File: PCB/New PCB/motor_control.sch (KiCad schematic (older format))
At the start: 29 parts, among them P4 CONN_2, P5 CONN_2, Q1 MOSFET_P, Q2 MOSFET_N, Q3 MOSFET_N, Q4 MOSFET_N, Q5 MOSFET_P, Q6 MOSFET_N, Q7 MOSFET_P, Q8 MOSFET_N, U4 MMPQ3904, U5 HEF4049B

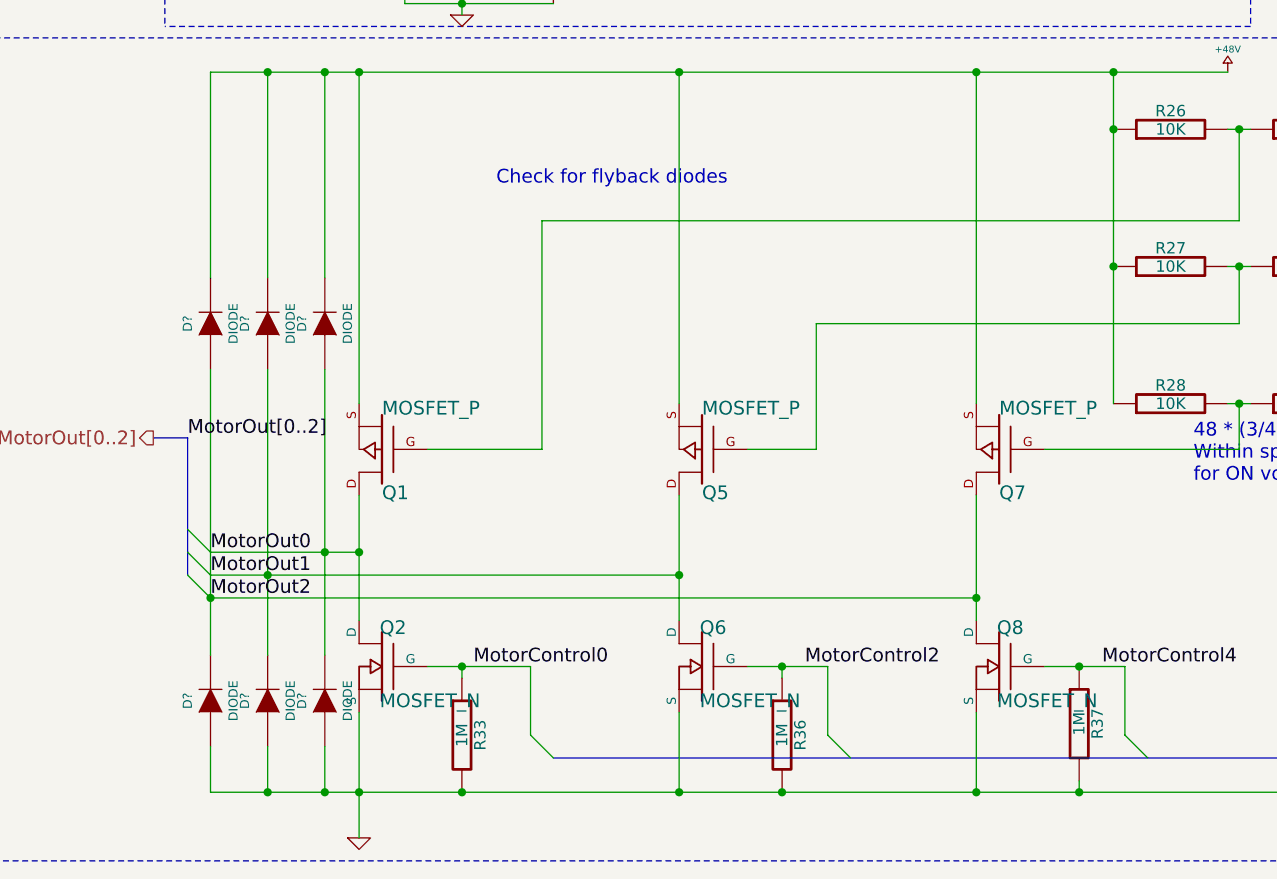
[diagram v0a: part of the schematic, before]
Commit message: order has been placed and confirmed, receipt in project folder
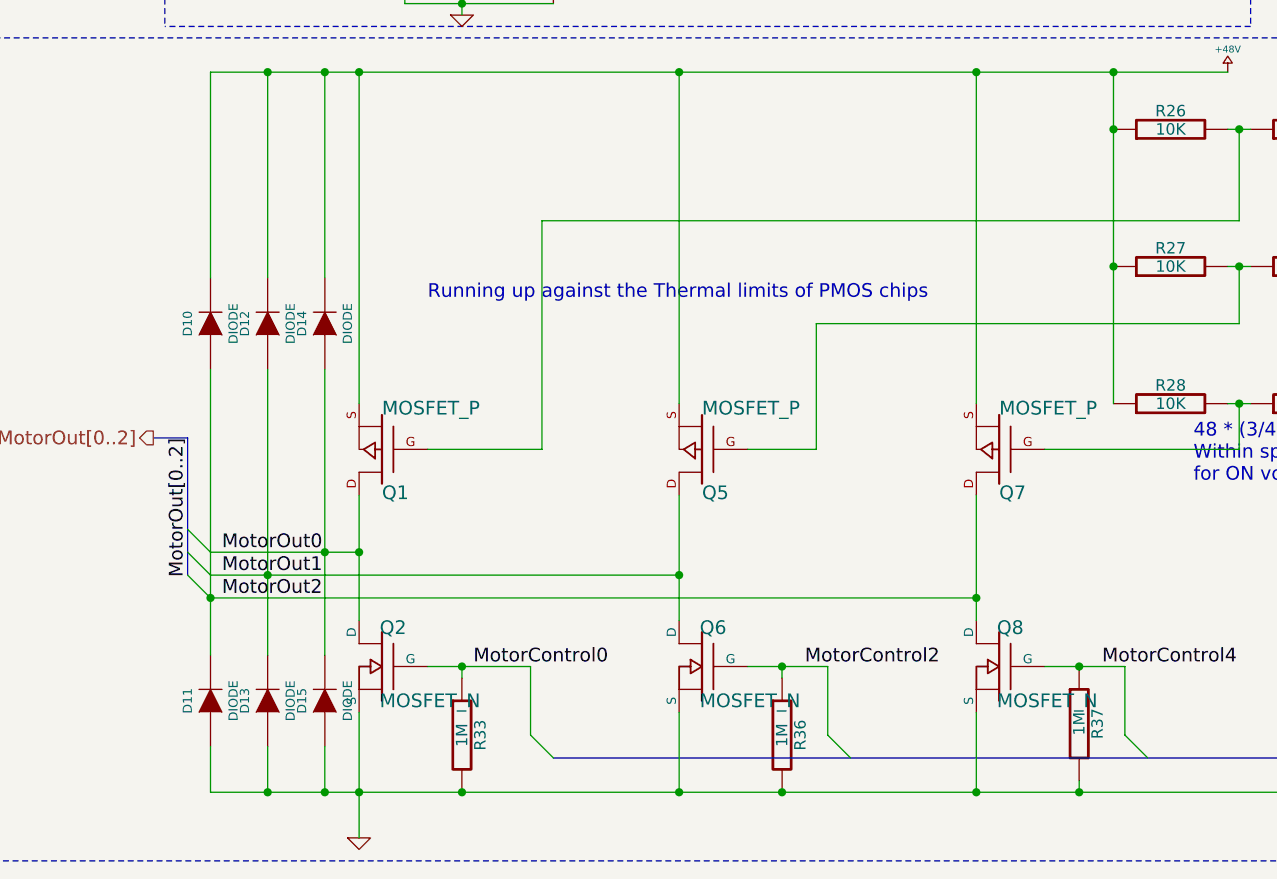
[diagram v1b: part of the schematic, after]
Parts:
- gave numbers to parts that had none: 6
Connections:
- net MotorOut0: no longer D10.1 (A), D11.2 (K), D12.1 (A), D13.2 (K), Q5.D, Q6.D, Q7.D, Q8.D
- new net MotorOut1: D12.1 (A), D13.2 (K), Q5.D, Q6.D
- new net MotorOut2: D10.1 (A), D11.2 (K), Q7.D, Q8.D
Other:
- note added: "Running up against the Thermal limits of PMOS chips"
- note removed: "Check for flyback diodes"
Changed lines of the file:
@@
 Sheet 3 4
 Title ""
-Date "3 jun 2013"
+Date "5 jun 2013"
 Rev ""
 Comp ""
@@
 Entry Wire Line
 	1350 5850 1450 5950
-Text Label 1450 5750 0    60   ~ 0
+Text Label 1500 5750 0    60   ~ 0
 MotorOut0
-Text Label 1450 5850 0    60   ~ 0
+Text Label 1500 5850 0    60   ~ 0
 MotorOut1
-Text Label 1450 5950 0    60   ~ 0
+Text Label 1500 5950 0    60   ~ 0
 MotorOut2
 $Comp
-L GND #PWR095
+L GND #PWR0101
 U 1 1 51A8E3D4
 P 2100 7000
-F 0 "#PWR095" H 2100 7000 30  0001 C CNN
+F 0 "#PWR0101" H 2100 7000 30  0001 C CNN
 F 1 "GND" H 2100 6930 30  0001 C CNN
 F 2 "" H 2100 7000 60  0000 C CNN
@@
 PMOS NOTE:\nSince typically a PMOS is driven with a\nlow voltage, and our circuit demands a \nhigh voltage to drive the resistor divider \nnetwork, we invert the signal to keep the\nlogic levels compatable.
 $Comp
-L +24V #PWR096
+L +24V #PWR0102
 U 1 1 51A90C79
 P 2050 1200
-F 0 "#PWR096" H 2050 1150 20  0001 C CNN
+F 0 "#PWR0102" H 2050 1150 20  0001 C CNN
 F 1 "+24V" H 2050 1300 30  0000 C CNN
 F 2 "" H 2050 1200 60  0000 C CNN
@@
 $EndComp
 $Comp
-L +24V #PWR097
+L +24V #PWR0103
 U 1 1 51A90C88
 P 2050 2300
-F 0 "#PWR097" H 2050 2250 20  0001 C CNN
+F 0 "#PWR0103" H 2050 2250 20  0001 C CNN
 F 1 "+24V" H 2050 2400 30  0000 C CNN
 F 2 "" H 2050 2300 60  0000 C CNN
@@
 $EndComp
 $Comp
-L +48V #PWR098
+L +48V #PWR0104
 U 1 1 51A90C97
 P 5900 3650
-F 0 "#PWR098" H 5900 3780 20  0001 C CNN
+F 0 "#PWR0104" H 5900 3780 20  0001 C CNN
 F 1 "+48V" H 5900 3750 30  0000 C CNN
 F 2 "" H 5900 3650 60  0000 C CNN
@@
 Text Label 3650 1500 0    60   ~ 0
 MagnetControl[0..1]
-Text Label 1350 5250 0    60   ~ 0
+Text Label 1350 5250 3    60   ~ 0
 MotorOut[0..2]
 Text Notes 9250 4950 0    60   ~ 0
 Double check initialization routine for fast PWM
-Text Notes 2700 4150 0    60   ~ 0
-Check for flyback diodes
 Text Label 2600 6250 0    60   ~ 0
 MotorControl0
@@
 $EndComp
 $Comp
-L GND #PWR099
+L GND #PWR0105
 U 1 1 51ABEB8A
 P 2750 2300
-F 0 "#PWR099" H 2750 2300 30  0001 C CNN
+F 0 "#PWR0105" H 2750 2300 30  0001 C CNN
 F 1 "GND" H 2750 2230 30  0001 C CNN
 F 2 "" H 2750 2300 60  0000 C CNN
@@
 $EndComp
 $Comp
-L GND #PWR0100
+L GND #PWR0106
 U 1 1 51ABED05
 P 2550 3400
-F 0 "#PWR0100" H 2550 3400 30  0001 C CNN
+F 0 "#PWR0106" H 2550 3400 30  0001 C CNN
 F 1 "GND" H 2550 3330 30  0001 C CNN
 F 2 "" H 2550 3400 60  0000 C CNN
@@
 $EndComp
 $Comp
-L VCC #PWR0101
+L VCC #PWR0107
 U 1 1 51AC138D
 P 8950 4200
-F 0 "#PWR0101" H 8950 4300 30  0001 C CNN
+F 0 "#PWR0107" H 8950 4300 30  0001 C CNN
 F 1 "VCC" H 8950 4300 30  0000 C CNN
 F 2 "" H 8950 4200 60  0000 C CNN
@@
 $EndComp
 $Comp
-L DIODE D?
+L DIODE D11
 U 1 1 51ACC20D
 P 1450 6400
-F 0 "D?" H 1450 6500 40  0000 C CNN
+F 0 "D11" H 1450 6500 40  0000 C CNN
 F 1 "DIODE" H 1450 6300 40  0000 C CNN
 F 2 "" H 1450 6400 60  0000 C CNN
@@
 $EndComp
 $Comp
-L DIODE D?
+L DIODE D13
 U 1 1 51ACC21A
 P 1700 6400
-F 0 "D?" H 1700 6500 40  0000 C CNN
+F 0 "D13" H 1700 6500 40  0000 C CNN
 F 1 "DIODE" H 1700 6300 40  0000 C CNN
 F 2 "" H 1700 6400 60  0000 C CNN
@@
 $EndComp
 $Comp
-L DIODE D?
+L DIODE D15
 U 1 1 51ACC220
 P 1950 6400
-F 0 "D?" H 1950 6500 40  0000 C CNN
+F 0 "D15" H 1950 6500 40  0000 C CNN
 F 1 "DIODE" H 1950 6300 40  0000 C CNN
 F 2 "" H 1950 6400 60  0000 C CNN
@@
 $EndComp
 $Comp
-L DIODE D?
+L DIODE D10
 U 1 1 51ACC59C
 P 1450 4750
-F 0 "D?" H 1450 4850 40  0000 C CNN
+F 0 "D10" H 1450 4850 40  0000 C CNN
 F 1 "DIODE" H 1450 4650 40  0000 C CNN
 F 2 "" H 1450 4750 60  0000 C CNN
@@
 $EndComp
 $Comp
-L DIODE D?
+L DIODE D12
 U 1 1 51ACC5A2
 P 1700 4750
-F 0 "D?" H 1700 4850 40  0000 C CNN
+F 0 "D12" H 1700 4850 40  0000 C CNN
 F 1 "DIODE" H 1700 4650 40  0000 C CNN
 F 2 "" H 1700 4750 60  0000 C CNN
@@
 $EndComp
 $Comp
-L DIODE D?
+L DIODE D14
 U 1 1 51ACC5A8
 P 1950 4750
-F 0 "D?" H 1950 4850 40  0000 C CNN
+F 0 "D14" H 1950 4850 40  0000 C CNN
 F 1 "DIODE" H 1950 4650 40  0000 C CNN
 F 2 "" H 1950 4750 60  0000 C CNN
@@
 Connection ~ 1700 3650
 Connection ~ 1950 3650
+Text Notes 2400 4650 0    60   ~ 0
+Running up against the Thermal limits of PMOS chips
 $EndSCHEMATC
